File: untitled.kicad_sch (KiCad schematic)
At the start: 17 parts, among them CN1 XT30PW-M, CN2 XT30PW-M, SW1 SWITCH_BLACK, SW2 SWITCH_BLACK, U14 XL4005, U15 XC6220B331MR

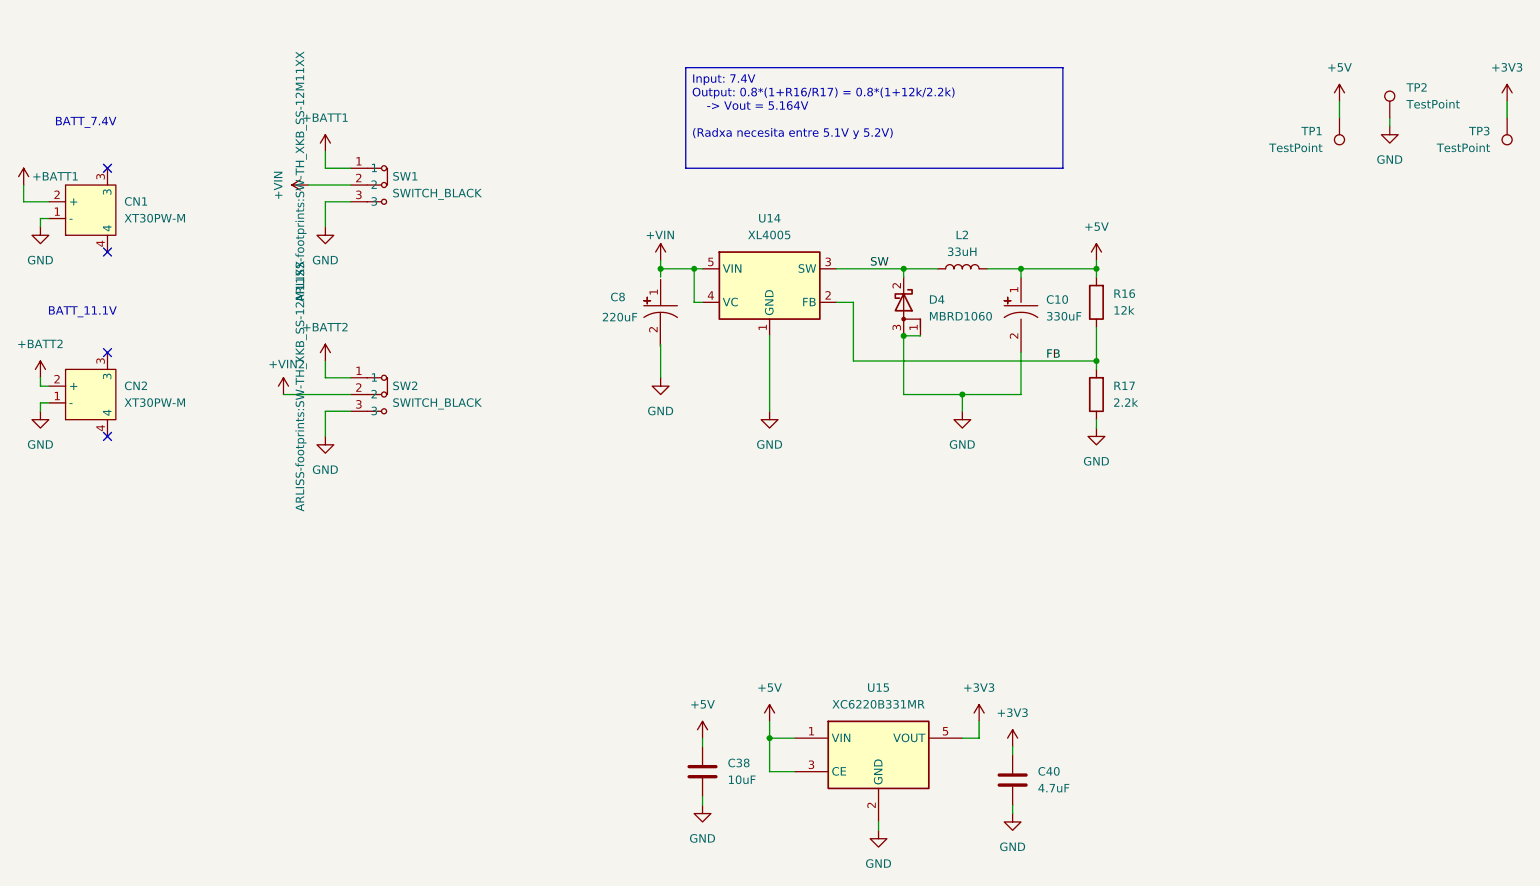
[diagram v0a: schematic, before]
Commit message: feat: [solución de rules checker]
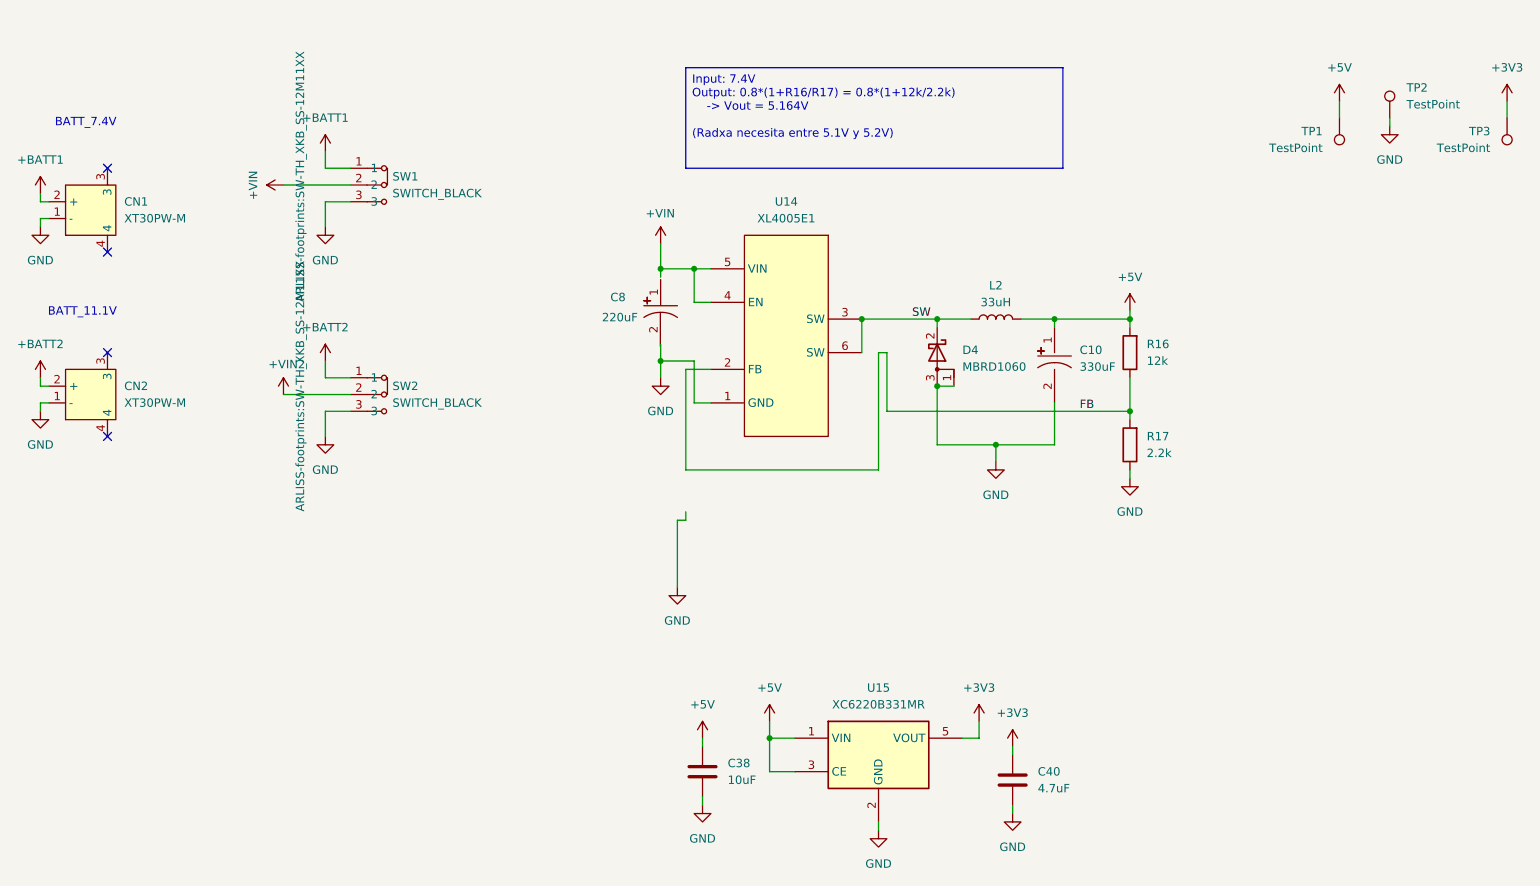
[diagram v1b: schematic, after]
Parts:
- removed U14: XL4005, Package_TO_SOT_SMD:TO-263-5_TabPin3, symbol Regulator_Switching:XL4015
- added U14: XL4005E1, easyeda2kicad:TO-263-5_L10.2-W9.2-P1.70-TL, symbol CANSAT_STM32_symbols:XL4005E1
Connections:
- net +VIN: now also U14.4 (EN), U14.5 (VIN)
- net FB: now also U14.2 (FB)
- net GND: now also U14.1 (GND)
- net SW: now also U14.3 (SW), U14.6 (SW)
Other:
- moved on the sheet: C10, D4, L2, R16, R17
